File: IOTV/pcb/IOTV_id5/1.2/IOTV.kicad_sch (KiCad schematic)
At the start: 24 parts, among them J1 Screw_Terminal_01x02, J2 Screw_Terminal_01x02, J3 Conn_01x04, J4 Conn_01x04, J5 Conn_01x04, J6 Conn_01x05, J8 UART, Q1 S8050, SW1 RST, SW2 Boot, U1 ESP32-WROOM-E, U2 G7DA-28 (Z)D3 8A/240V (3-32V)

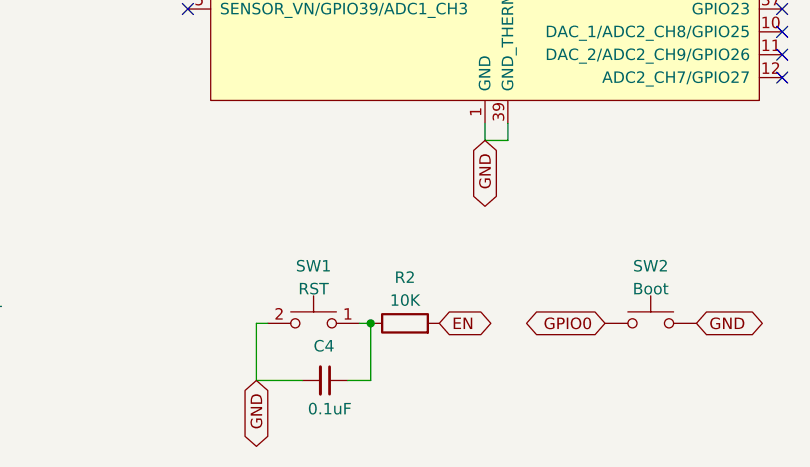
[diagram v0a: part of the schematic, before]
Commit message: pcb id5
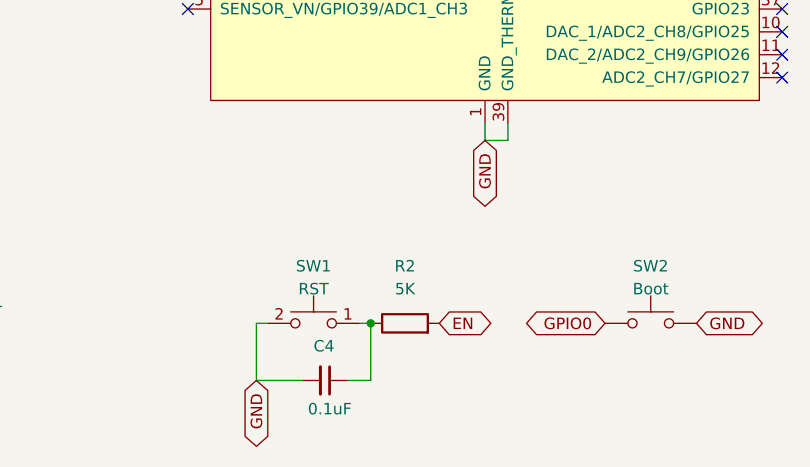
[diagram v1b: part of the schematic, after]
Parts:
- R2: value 10K -> 5K
